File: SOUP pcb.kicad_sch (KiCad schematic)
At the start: 24 parts, among them J1 Conn_01x06_Pin, J2 Conn_01x02, J3 Conn_01x02, SW1 SW_SPST, SW2 SW_Push, SW3 SW_Push, SW4 SW_Push, U1 ESP32-WROOM-32, U2 MAX98357A, U3 AP2112K-3.3

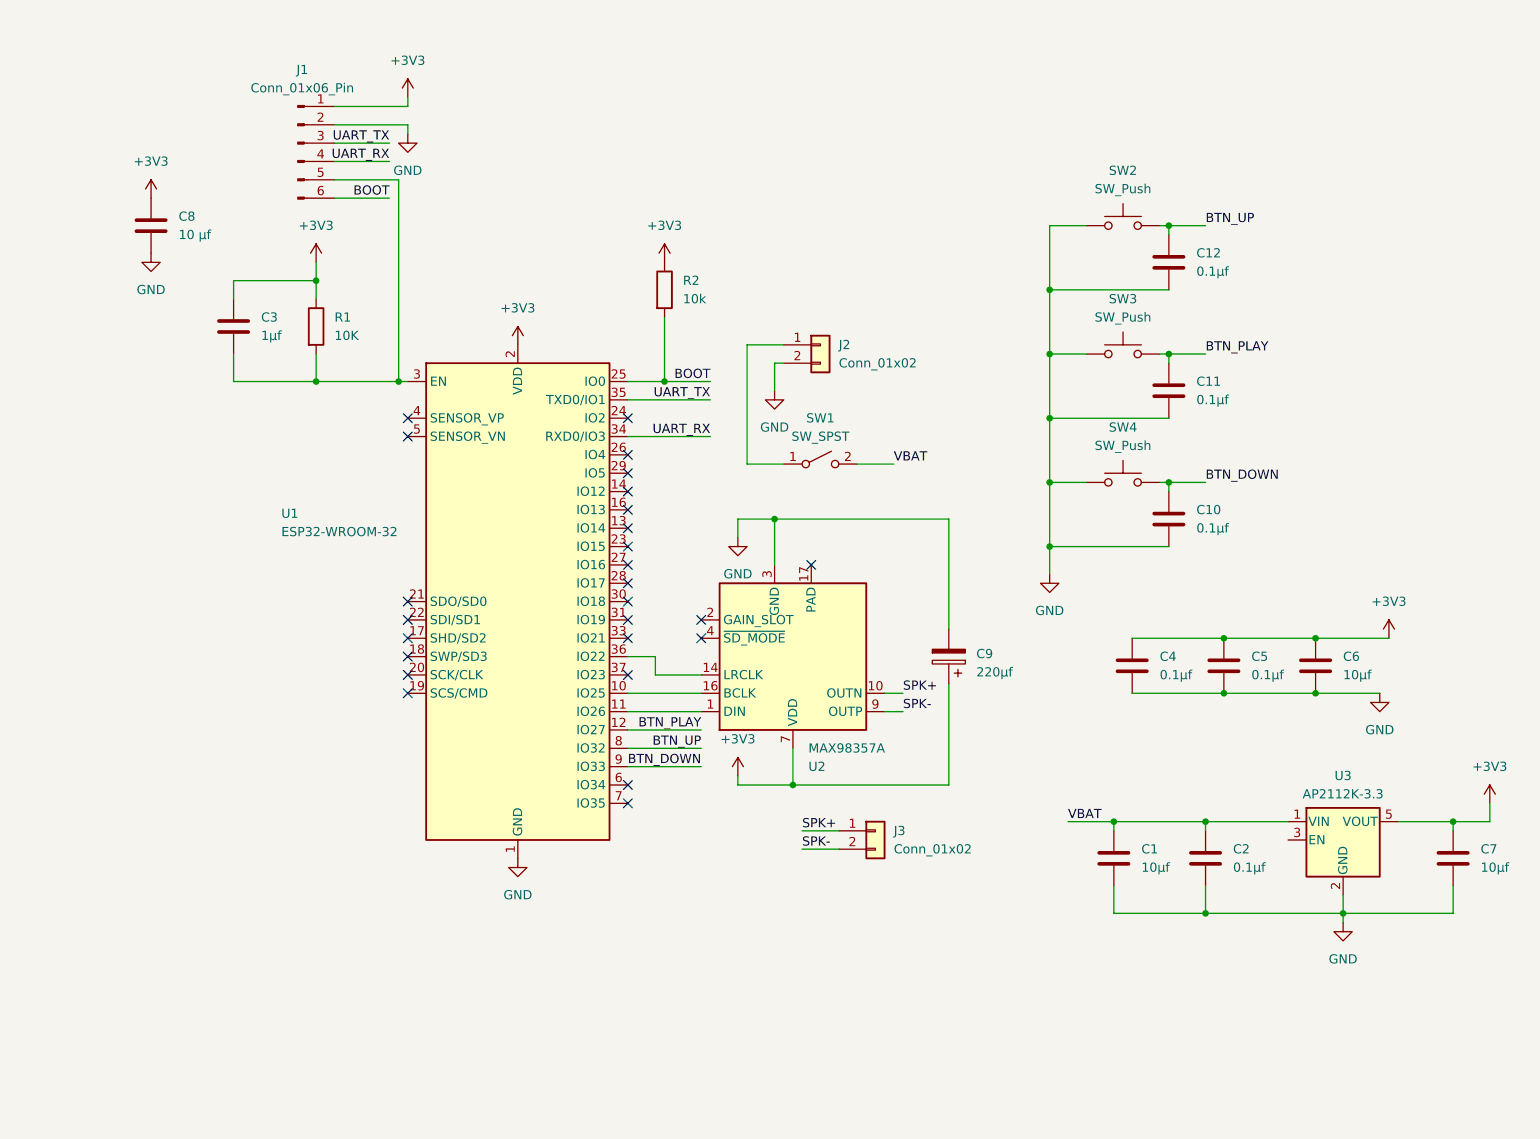
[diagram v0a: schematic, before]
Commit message: Add files via upload
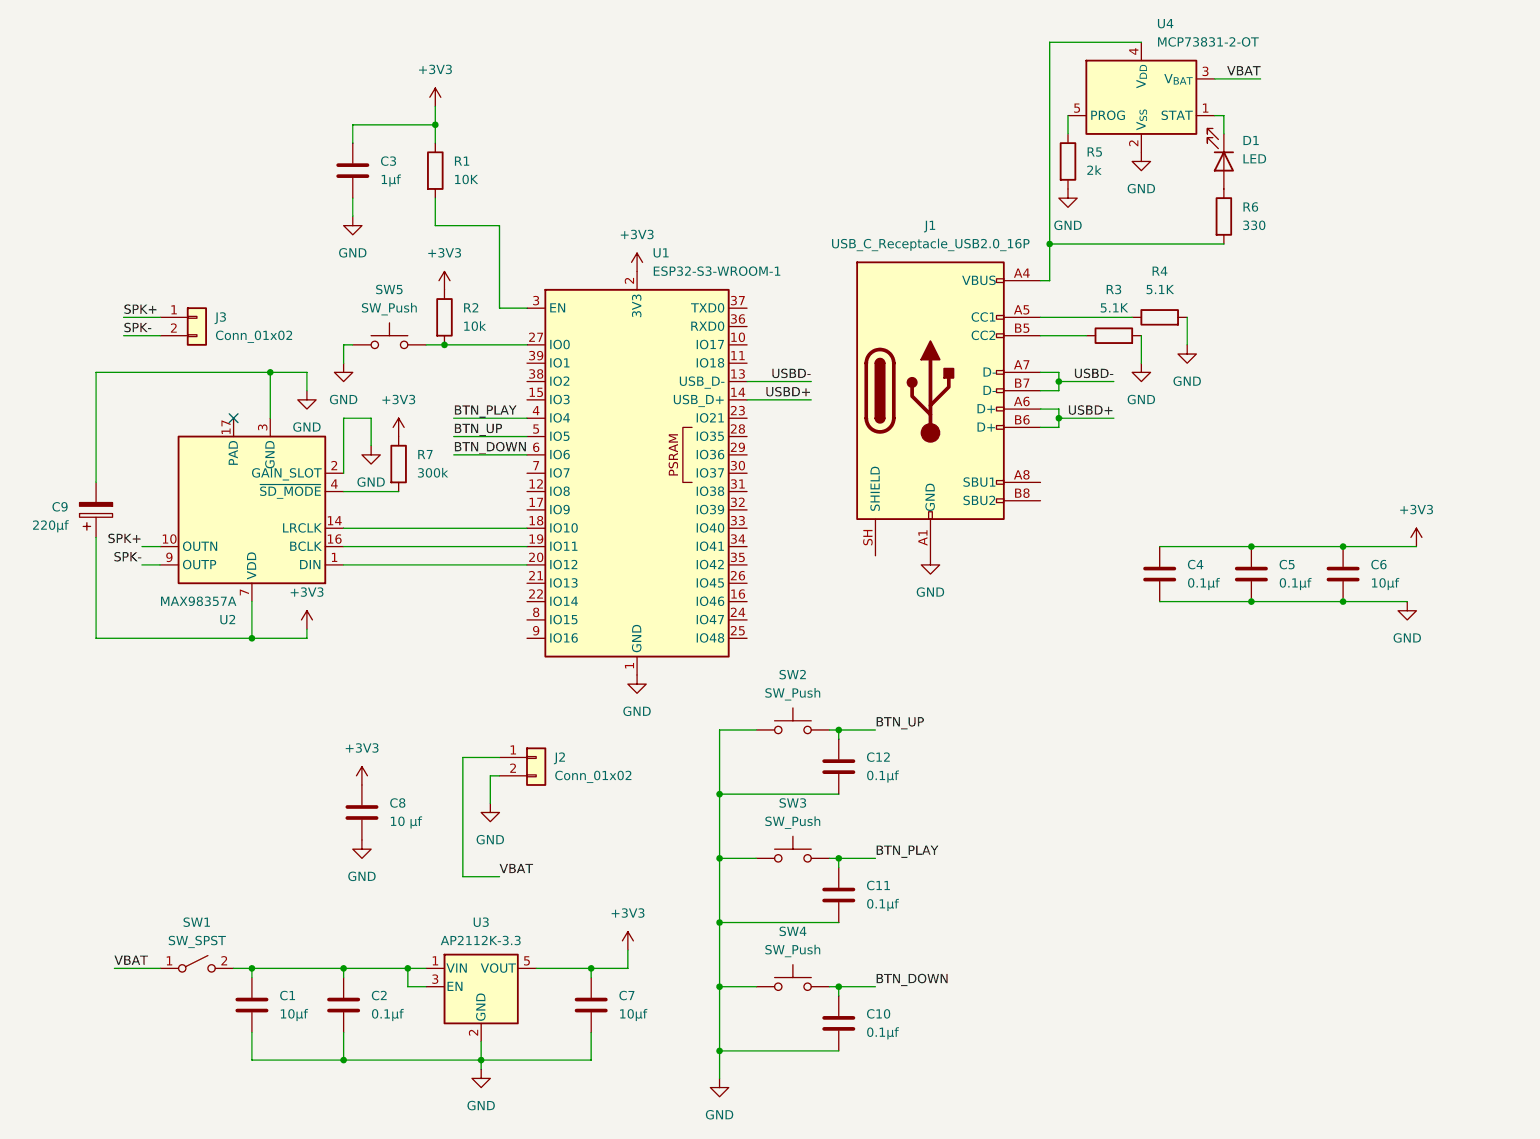
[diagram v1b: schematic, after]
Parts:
- removed J1: Conn_01x06_Pin, Connector_PinHeader_2.54mm:PinHeader_1x06_P2.54mm_Vertical, symbol Connector:Conn_01x06_Pin
- removed U1: ESP32-WROOM-32, RF_Module:ESP32-WROOM-32, symbol RF_Module:ESP32-WROOM-32
- added D1: LED, LED_SMD:LED_0603_1608Metric, symbol Device:LED
- added J1: USB_C_Receptacle_USB2.0_16P, Connector_USB:USB_C_Receptacle_HRO_TYPE-C-31-M-12, symbol Connector:USB_C_Receptacle_USB2.0_16P
- added R3, R4: 5.1K, Resistor_SMD:R_0603_1608Metric, symbol Device:R
- added R5: 2k, Resistor_SMD:R_0603_1608Metric, symbol Device:R
- added R6: 330, Resistor_SMD:R_0603_1608Metric, symbol Device:R
- added R7: 300k, Resistor_SMD:R_0603_1608Metric, symbol Device:R
- added SW5: SW_Push, Button_Switch_SMD:SW_SPST_PTS645Sx43SMTR92, symbol Switch:SW_Push
- added U1: ESP32-S3-WROOM-1, RF_Module:ESP32-S3-WROOM-1, symbol RF_Module:ESP32-S3-WROOM-1
- added U4: MCP73831-2-OT, Package_TO_SOT_SMD:SOT-23-5, symbol Battery_Management:MCP73831-2-OT
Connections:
- net +3V3: now also R7.1, U1.2 (3V3)
- net BTN_DOWN: now also U1.6 (IO6)
- net BTN_PLAY: now also U1.4 (IO4)
- net BTN_UP: now also U1.5 (IO5)
- net GND: now also C3.2, U2.2 (GAIN_SLOT), J1.A1 (GND), J1.A12 (GND), J1.B1 (GND), J1.B12 (GND), R3.2, R4.2, R5.2, SW5.1, U1.1 (GND), U1.40 (GND), U1.41 (GND), U4.2 (V_{SS})
- net VBAT: now also J2.1 (Pin_1), SW1.1 (A), U4.3 (V_{BAT}); no longer C1.1, C2.1, SW1.2 (B), U3.1 (VIN)
- net at U2.16 (BCLK): now also U1.19 (IO11)
- net at U2.1 (DIN): now also U1.20 (IO12)
- net at R1.2: now also U1.3 (EN); no longer C3.2
- net at U2.14 (LRCLK): now also U1.18 (IO10)
- net at U3.3 (EN): now also C1.1, C2.1, SW1.2 (B), U3.1 (VIN)
- net at U2.4 (~{SD_MODE}): now also R7.2
- net BOOT: no longer names the net of R2.2
- net BOOT: now also SW5.2, U1.27 (IO0)
- new net: J1.A5 (CC1), R4.1
- new net: R5.1, U4.5 (PROG)
- new net: D1.1 (K), U4.1 (STAT)
- new net: J1.A4 (VBUS), J1.A9 (VBUS), J1.B4 (VBUS), J1.B9 (VBUS), R6.2, U4.4 (V_{DD})
- new net: J1.B5 (CC2), R3.1
- new net: D1.2 (A), R6.1
- new net USBD+: J1.A6 (D+), J1.B6 (D+), U1.14 (USB_D+)
- new net USBD-: J1.A7 (D-), J1.B7 (D-), U1.13 (USB_D-)
- no-connect marks 26 -> 1
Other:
- moved on the sheet: C1, C10, C11, C12, C2, C3, C4, C5, C6, C7, C8, C9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
